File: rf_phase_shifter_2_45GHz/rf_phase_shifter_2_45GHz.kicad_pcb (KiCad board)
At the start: 2 copper layers, 12 parts, among them J1 CON-SMA-EDGE-S, J2 CON-SMA-EDGE-S, J3 CON-SMA-EDGE-S

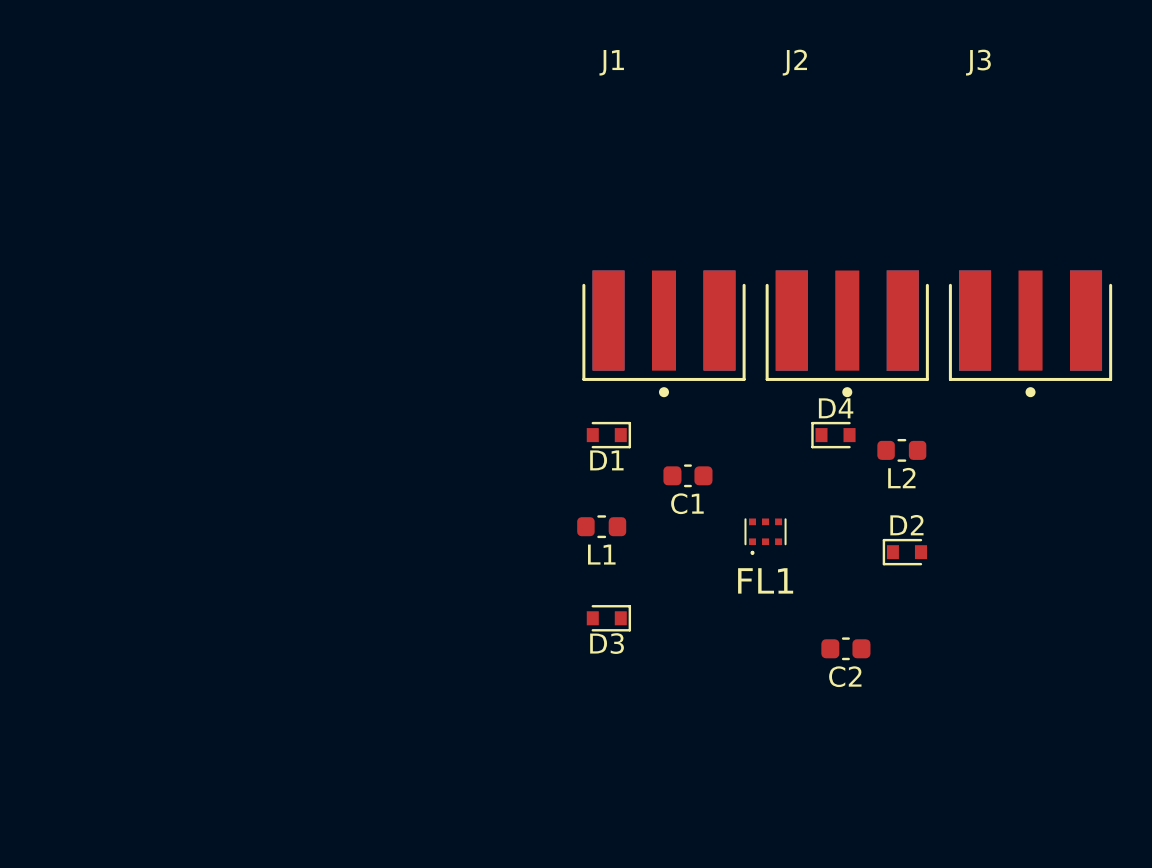
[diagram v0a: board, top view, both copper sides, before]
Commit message: finished pcb layouts
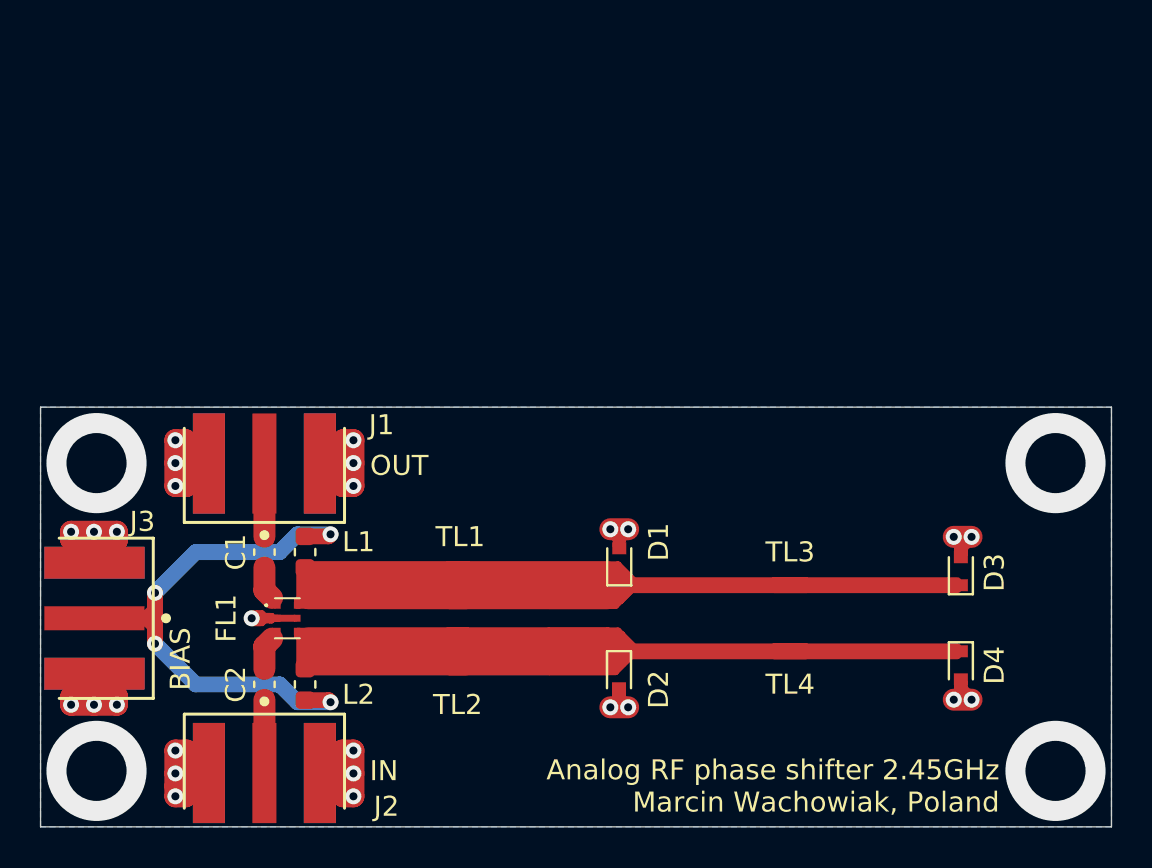
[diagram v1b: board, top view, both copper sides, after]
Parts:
- added TL1: TL_13_2_45GHz, analog_rf_phase_shifter_module:TL_13_2_45GHz, F.Cu at (94.1, 57.3)
- added TL2: TL_13_2_45GHz, analog_rf_phase_shifter_module:TL_13_2_45GHz, F.Cu at (94.1, 60.6)
- added TL3: TL_24_2_45GHz, analog_rf_phase_shifter_module:TL_24_2_45GHz, F.Cu at (110.7, 57.3)
- added TL4: TL_24_2_45GHz, analog_rf_phase_shifter_module:TL_24_2_45GHz, F.Cu at (110.7, 60.6)
- moved J3 58.4 mm to (68.7, 58.9), turned to 90 degrees
- moved J2 47.2 mm to (84.5, 73.9), turned to 180 degrees
- moved L2 32.0 mm to (86.5, 62.2), turned to 90 degrees
- moved C2 29.1 mm to (84.5, 62.2), turned to 90 degrees
- moved FL1 24.3 mm to (85.6, 58.9), turned to 270 degrees
- moved C1 21.5 mm to (84.5, 55.6), turned to 90 degrees
- moved J1 21.2 mm to (84.5, 43.9)
- moved D3 17.8 mm to (119.2, 56.6), turned to 90 degrees
- moved D2 15.6 mm to (102.2, 61.7), turned to 270 degrees
- moved L1 14.9 mm to (86.5, 55.6), turned to 270 degrees
- moved D4 13.1 mm to (119.2, 61.3), turned to 270 degrees
- moved D1 6.38 mm to (102.2, 56.1), turned to 90 degrees
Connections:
- D3 pad 1: Net-(D1-Pad1) -> Net-(D3-Pad1)
- D4 pad 1: Net-(D2-Pad1) -> Net-(D4-Pad1)
- FL1 pad 4: Net-(D2-Pad1) -> Net-(FL1-Pad4)
- FL1 pad 6: Net-(D1-Pad1) -> Net-(FL1-Pad6)
- L1 pad 2: Net-(D1-Pad1) -> Net-(FL1-Pad6)
- L2 pad 2: Net-(D2-Pad1) -> Net-(FL1-Pad4)
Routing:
- net GND: track 0.00 -> 69.4 mm, vias 0 -> 31
- net Net-(D2-Pad1): track 0.00 -> 46.8 mm
- net Net-(J3-Pad1): track 0.00 -> 30.7 mm, vias 0 -> 4
- net Net-(D1-Pad1): track 0.00 -> 30.5 mm
- net Net-(FL1-Pad4): track 0.00 -> 9.93 mm
- net Net-(D4-Pad1): track 0.00 -> 8.48 mm
- net Net-(FL1-Pad6): track 0.00 -> 6.22 mm
- net Net-(D3-Pad1): track 0.00 -> 4.75 mm
- net Net-(C1-Pad2): track 0.00 -> 3.65 mm
- net Net-(C2-Pad1): track 0.00 -> 3.65 mm
- net Net-(C2-Pad2): track 0.00 -> 1.67 mm
- net Net-(C1-Pad1): track 0.00 -> 1.67 mm
- added copper zone on B.Cu, net GND
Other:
- board outline added: 53.5 x 21 mm
- board text added: "Analog RF phase shifter 2.45GHz Marcin Wachowiak, Poland"
- board text added: "BIAS"
- board text added: "IN"
- board text added: "OUT"
